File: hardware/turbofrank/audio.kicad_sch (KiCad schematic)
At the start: 13 parts

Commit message: TurboFRANK HW 1.03
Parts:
- TDA1: footprint FRANK:SOIC-8 -> FRANK:SO-8
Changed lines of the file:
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@@
 		(title "TurboFRANK")
 		(date "2025-03-03")
-		(rev "1.02")
+		(rev "1.03")
 		(company "Mikhail Matveev")
 		(comment 1 "https://github.com/xtremespb/frank")
@@
 			)
 		)
-		(property "Footprint" "FRANK:SOIC-8"
+		(property "Footprint" "FRANK:SO-8"
 			(at 186.69 59.69 0)
 			(effects

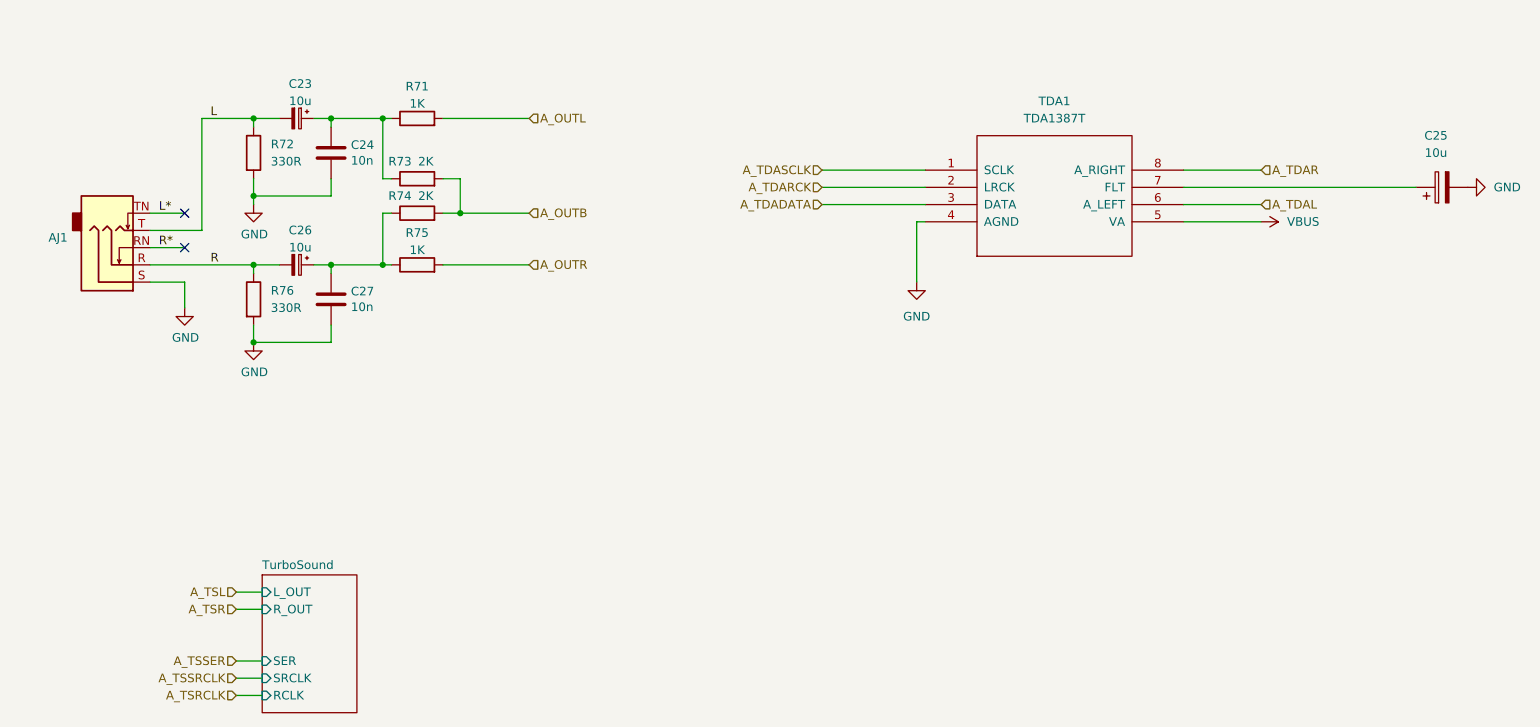
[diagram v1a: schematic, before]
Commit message: TurboFRANK 1.04 WIP
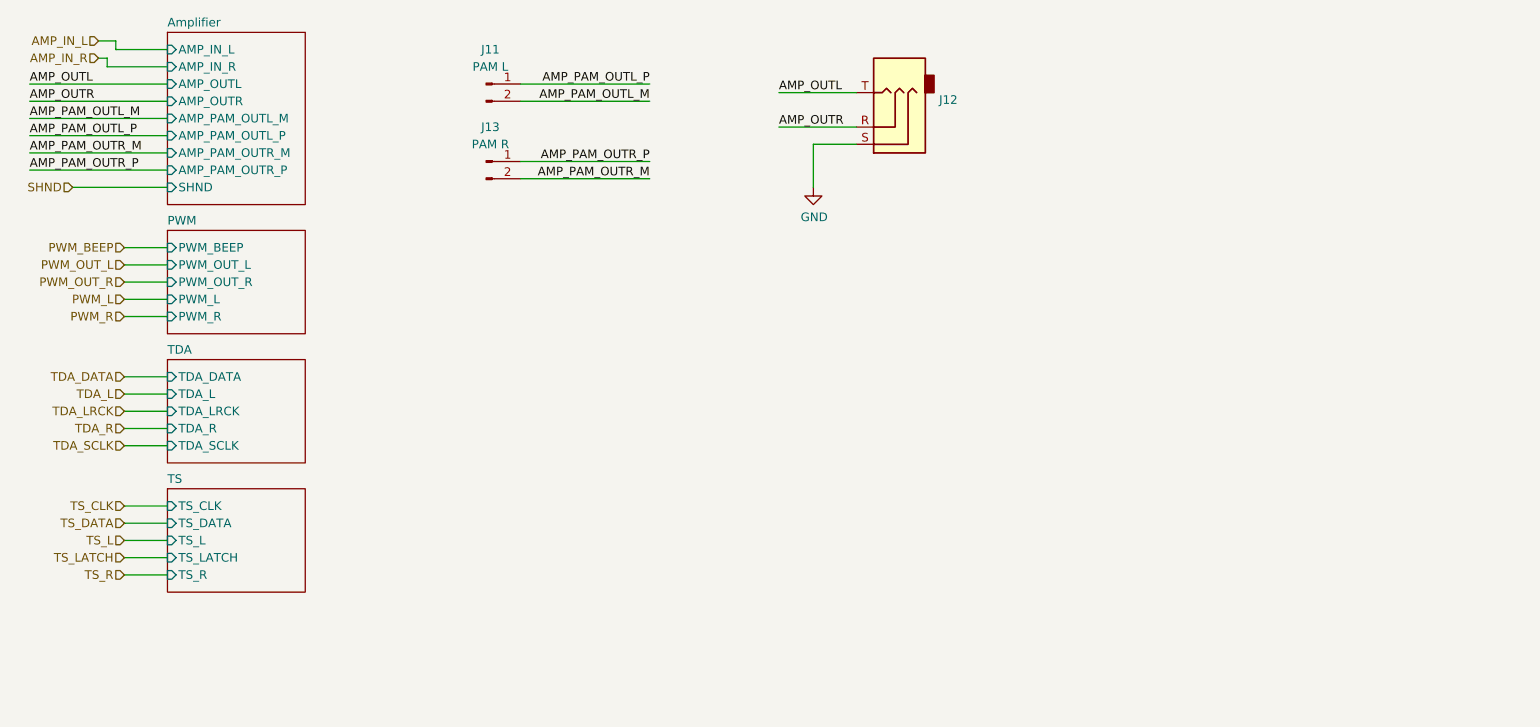
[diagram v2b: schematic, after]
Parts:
- removed C23, C26: 10u, FRANK:Capacitor (3528, tantalum, polar), symbol Device:C_Polarized_Small
- removed C24, C27: 10n, FRANK:Capacitor (0805), symbol Device:C
- removed C25: 10u, FRANK:Capacitor (3528, tantalum, polar), symbol Device:C_Polarized
- removed R71, R75: 1K, FRANK:Resistor (0805), symbol Device:R
- removed R72, R76: 330R, FRANK:Resistor (0805), symbol Device:R
- removed R73, R74: 2K, FRANK:Resistor (0805), symbol Device:R
- removed TDA1: TDA1387T, FRANK:SO-8, symbol FRANK:TDA1387T
- added J11: PAM L, FRANK:Connector Female ZH 1.50mm (2 pins), symbol Connector:Conn_01x02_Pin
- added J13: PAM R, FRANK:Connector Female ZH 1.50mm (2 pins), symbol Connector:Conn_01x02_Pin
- J12: renamed from AJ1; value SJ1-353XNG -> ~; footprint FRANK:Jack (3.5mm) -> FRANK:Jack (3.5mm, PJ-320D); AliExpress https://www.aliexpress.com/item/1005006710837751.html -> (none)
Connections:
- net L renamed AMP_OUTL
- removed net L*: J12.TN
- net R renamed AMP_OUTR
- removed net R*: J12.RN
- new net AMP_PAM_OUTL_M: J11.2 (Pin_2)
- new net AMP_PAM_OUTL_P: J11.1 (Pin_1)
- new net AMP_PAM_OUTR_M: J13.2 (Pin_2)
- new net AMP_PAM_OUTR_P: J13.1 (Pin_1)
- no-connect marks 2 -> 0
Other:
- removed sheet TurboSound
- added sheet Amplifier (amp.kicad_sch)
- added sheet PWM (pwm.kicad_sch)
- added sheet TDA (tda.kicad_sch)
- added sheet TS (ts.kicad_sch)
